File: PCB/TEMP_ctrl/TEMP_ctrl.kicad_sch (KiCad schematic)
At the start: 42 parts, among them J1 CH1, J2 CH2, J3 CH3, J4 CH4, J5 Conn_01x07_Pin, J6 Conn_01x07_Pin, Q3 DMN2056U, U1 LMC6484, U2 102010388, U3 AP2112K-3.3, U4 LMC6484

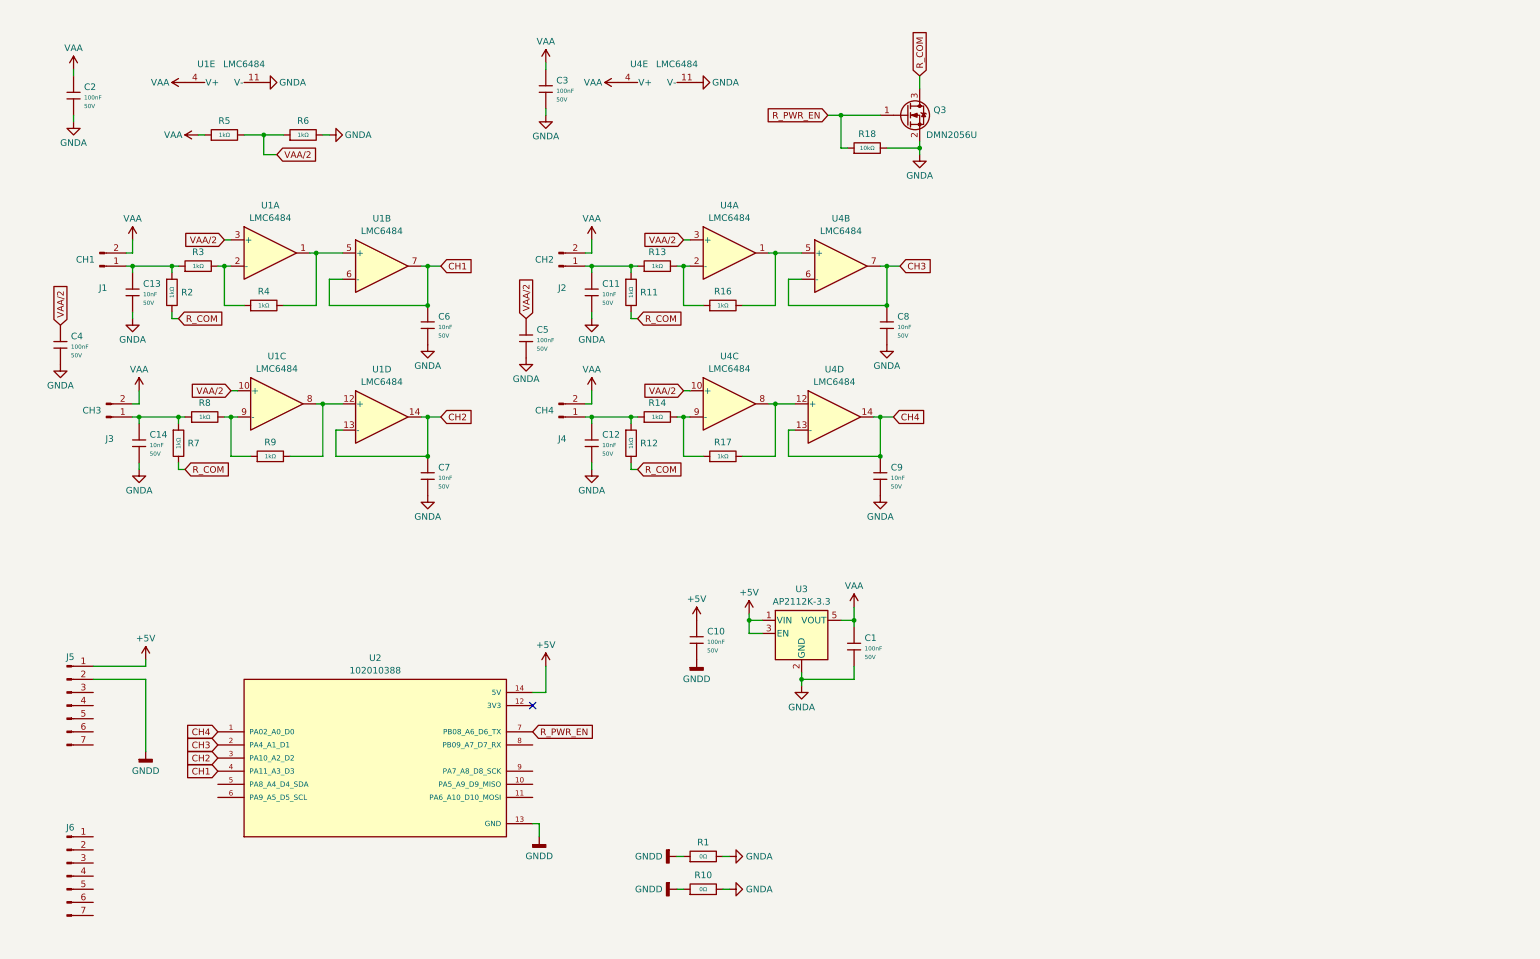
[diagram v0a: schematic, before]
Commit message: mac: finished PCB design
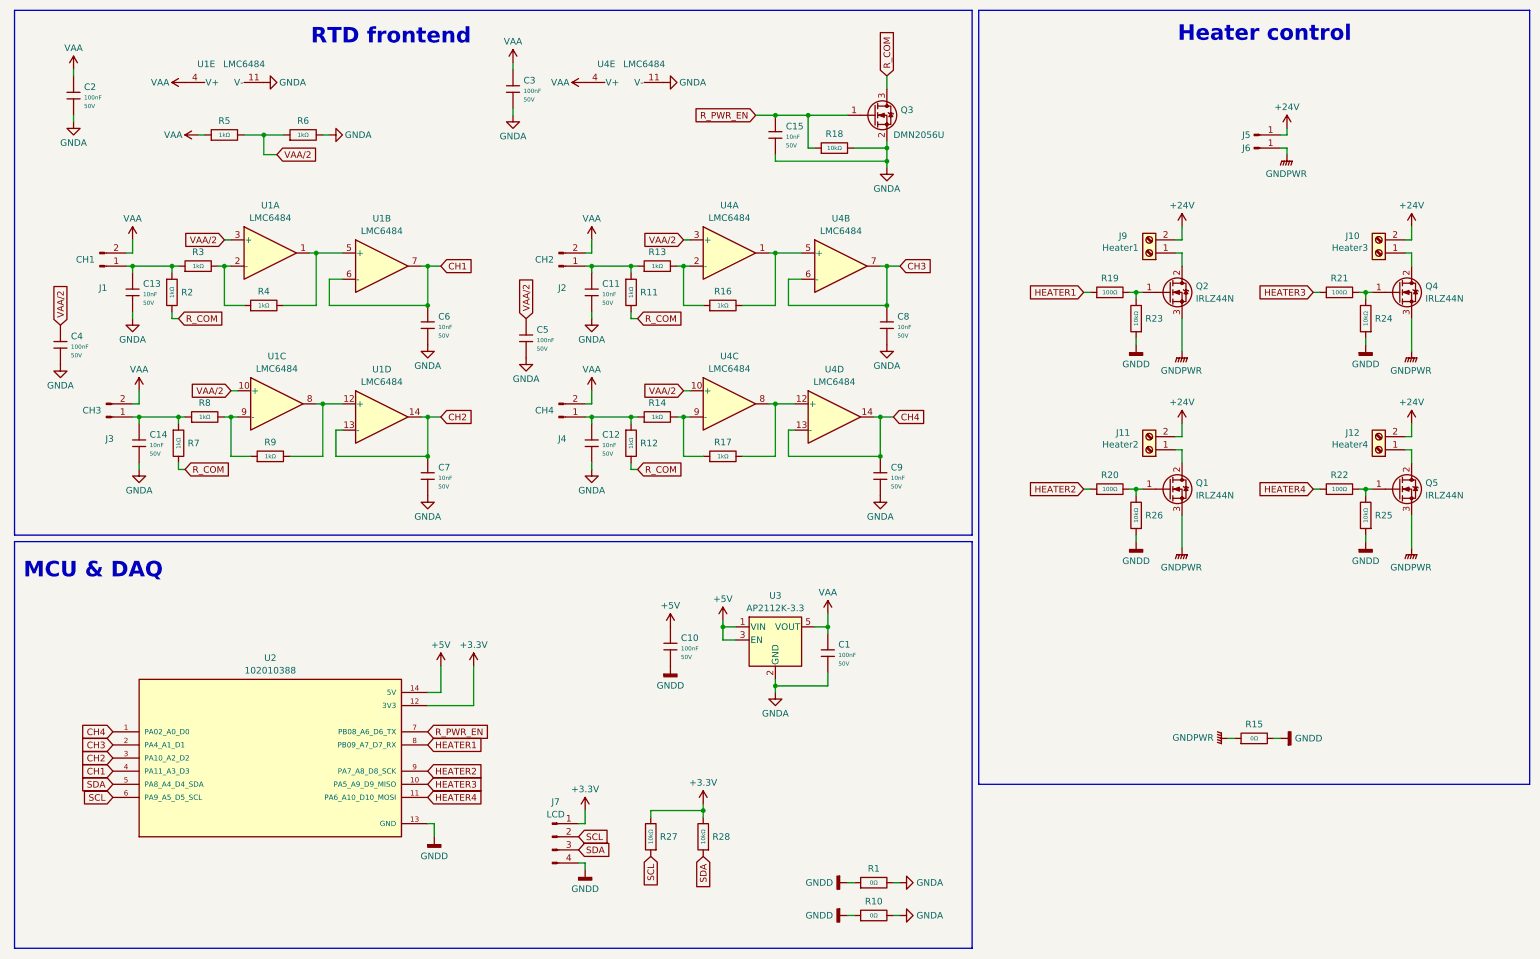
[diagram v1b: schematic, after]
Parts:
- removed J5, J6: Conn_01x07_Pin, symbol Connector:Conn_01x07_Pin
- added C15: 10nF, PCM_JLCPCB:C_1206, symbol PCM_JLCPCB-Capacitors:1206,100nF
- added J10: Heater3, TerminalBlock:TerminalBlock_MaiXu_MX126-5.0-02P_1x02_P5.00mm, symbol Connector:Screw_Terminal_01x02
- added J11: Heater2, TerminalBlock:TerminalBlock_MaiXu_MX126-5.0-02P_1x02_P5.00mm, symbol Connector:Screw_Terminal_01x02
- added J12: Heater4, TerminalBlock:TerminalBlock_MaiXu_MX126-5.0-02P_1x02_P5.00mm, symbol Connector:Screw_Terminal_01x02
- added J5, J6: Conn_01x01_Pin, TestPoint:TestPoint_Pad_4.0x4.0mm, symbol Connector:Conn_01x01_Pin
- added J7: LCD, Connector_PinHeader_2.54mm:PinHeader_1x04_P2.54mm_Vertical, symbol Connector:Conn_01x04_Pin
- added J9: Heater1, TerminalBlock:TerminalBlock_MaiXu_MX126-5.0-02P_1x02_P5.00mm, symbol Connector:Screw_Terminal_01x02
- added Q1, Q2, Q4, Q5: IRLZ44N, Package_TO_SOT_THT:TO-220-3_Vertical, symbol Transistor_FET:IRLZ44N
- added R15: 0Ω, PCM_JLCPCB:R_1206, symbol PCM_JLCPCB-Resistors:1206,0Ω
- added R19, R20, R21, R22: 100Ω, PCM_JLCPCB:R_1206, symbol PCM_JLCPCB-Resistors:1206,1kΩ
- added R23, R24, R25, R26, R27, R28: 10kΩ, PCM_JLCPCB:R_1206, symbol PCM_JLCPCB-Resistors:1206,1kΩ
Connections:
- net GNDA: now also C15.2
- net GNDD: now also J7.4 (Pin_4), R15.2, R23.1, R24.1, R25.1, R26.1
- net R_PWR_EN: now also C15.1
- net HEATER3: now reaches U2.10 (PA5_A9_D9_MISO)
- net HEATER3: now also R21.1
- net HEATER4: now reaches U2.11 (PA6_A10_D10_MOSI)
- net HEATER4: now also R22.1
- net +3.3V: now reaches U2.12 (3V3)
- net +3.3V: now also J7.1 (Pin_1), R27.2, R28.2
- net SDA: now reaches U2.5 (PA8_A4_D4_SDA)
- net SDA: now also J7.3 (Pin_3), R28.1
- net SCL: now reaches U2.6 (PA9_A5_D5_SCL)
- net SCL: now also J7.2 (Pin_2), R27.1
- net HEATER1: now reaches U2.8 (PB09_A7_D7_RX)
- net HEATER1: now also R19.1
- net HEATER2: now reaches U2.9 (PA7_A8_D8_SCK)
- net HEATER2: now also R20.1
- new net: Q2.1 (G), R19.2, R23.2
- new net: J9.1 (Pin_1), Q2.2 (D)
- new net: Q4.1 (G), R21.2, R24.2
- new net: J12.1 (Pin_1), Q5.2 (D)
- new net: Q5.1 (G), R22.2, R25.2
- new net: Q1.1 (G), R20.2, R26.2
- new net: J10.1 (Pin_1), Q4.2 (D)
- new net: J11.1 (Pin_1), Q1.2 (D)
- new net +24V: J10.2 (Pin_2), J11.2 (Pin_2), J12.2 (Pin_2), J5.1 (Pin_1), J9.2 (Pin_2)
- new net GNDPWR: J6.1 (Pin_1), Q1.3 (S), Q2.3 (S), Q4.3 (S), Q5.3 (S), R15.1
- no-connect marks 1 -> 0
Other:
- note added: "Heater control"
- note added: "MCU & DAQ"
- note added: "RTD frontend"
- moved on the sheet: C1, C10, C3, Q3, R1, R10, R18, U2, U3, U4E
